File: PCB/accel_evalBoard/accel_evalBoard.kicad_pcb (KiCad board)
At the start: 2 copper layers, 10 parts, among them J1 Conn_02x03_Odd_Even, J4 Conn_01x01

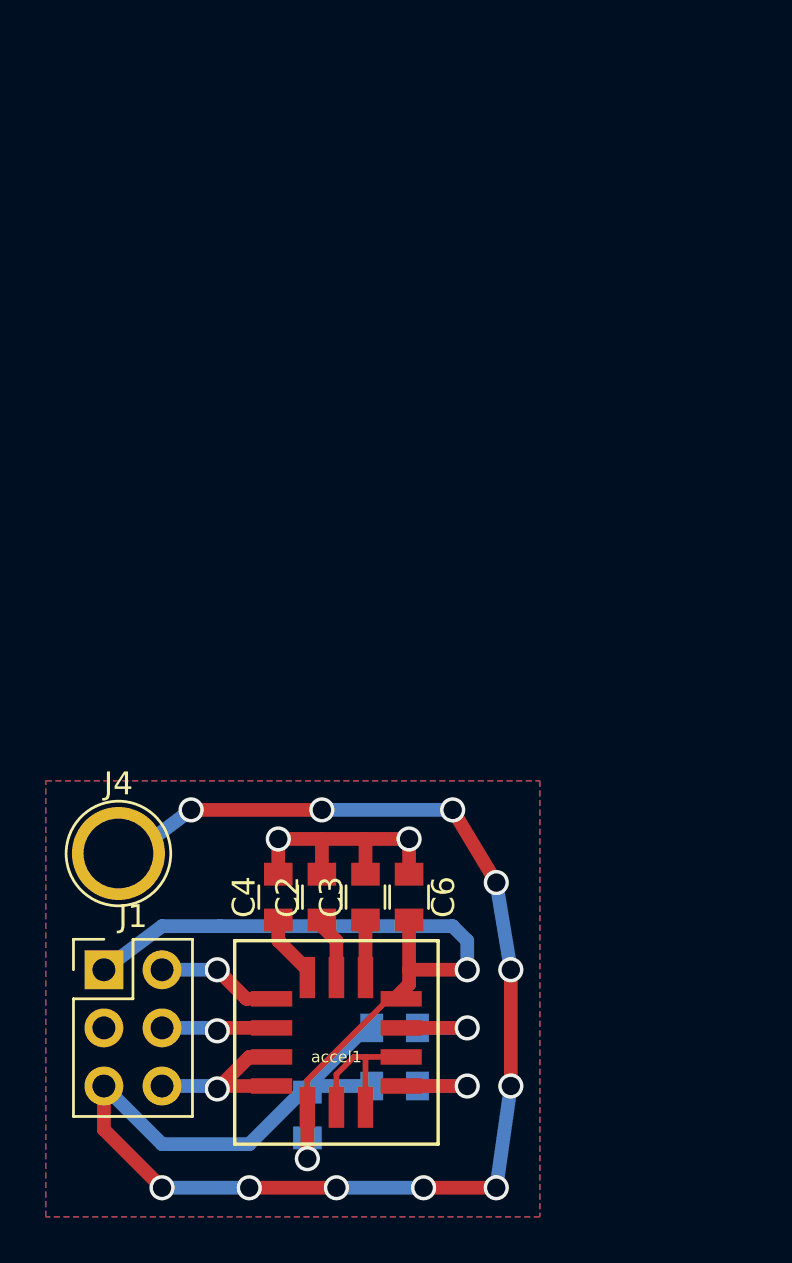
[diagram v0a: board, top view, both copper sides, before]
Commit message: Add PCB 2.3
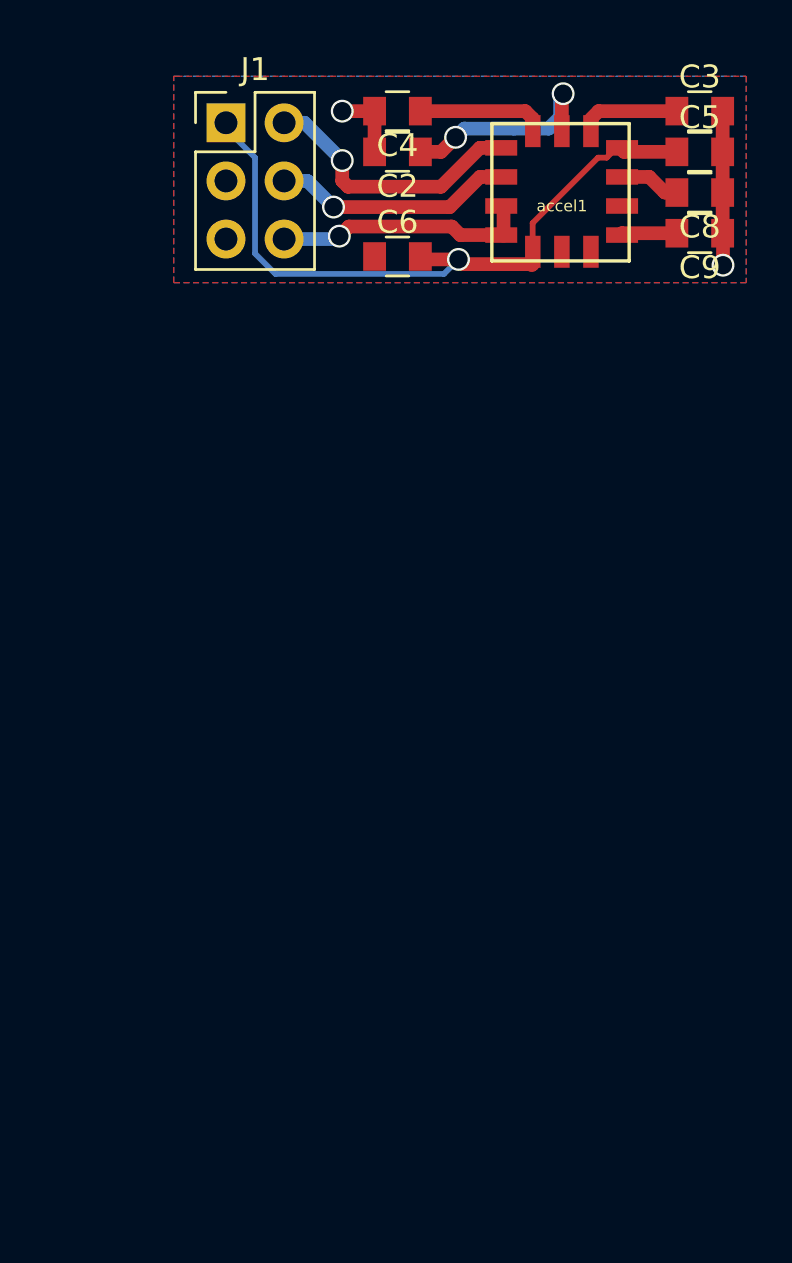
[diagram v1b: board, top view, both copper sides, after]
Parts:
- removed J4: Conn_01x01, Connectors:1pin
- C5, C8, C9: moved to F.Cu
- moved C5 45.4 mm to (186.7, 67.1), turned to 0 degrees
- moved C9 39.6 mm to (186.7, 70.7), turned to 180 degrees
- moved C8 38.9 mm to (186.7, 68.9), turned to 180 degrees
- moved J1 37.4 mm to (166.0, 65.9)
- moved C3 37.3 mm to (186.7, 65.4), turned to 0 degrees
- moved C4 34.7 mm to (173.5, 65.4), turned to 180 degrees
- moved C2 32.7 mm to (173.5, 67.1), turned to 180 degrees
- moved accel1 32.2 mm to (175.0, 74.5)
- moved C6 28.0 mm to (173.5, 71.7), turned to 0 degrees
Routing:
- net GNDREF: track 89.3 -> 9.93 mm, vias 13 -> 2
- net Net-(J1-Pad2): track 5.61 -> 12.2 mm
- net Net-(C2-Pad1): track 2.44 -> 8.93 mm, vias 0 -> 2
- net Net-(J1-Pad4): track 5.19 -> 10.6 mm
- net VDD: track 33.9 -> 30.4 mm, vias 2 -> 1
- net Net-(C9-Pad2): track 5.35 -> 2.52 mm, vias 1 -> 0
- net Net-(J1-Pad6): track 8.43 -> 11.2 mm
- net Net-(C8-Pad2): track 5.35 -> 2.77 mm, vias 1 -> 0
- net Net-(C4-Pad1): track 2.70 -> 5.06 mm
- net Net-(C3-Pad1): track 2.18 -> 3.89 mm
